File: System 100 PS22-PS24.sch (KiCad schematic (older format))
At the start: 39 parts, among them P1 CONN_01X01, P10 CONN_01X04, P11 CONN_01X06, P13 CONN_01X04, P2 CONN_01X01, P3 CONN_01X01, P4 CONN_01X01, P5 CONN_01X08, Q101 TIP31A, Q102 TIP31A, U101 LM723CN, U102 LM723CN

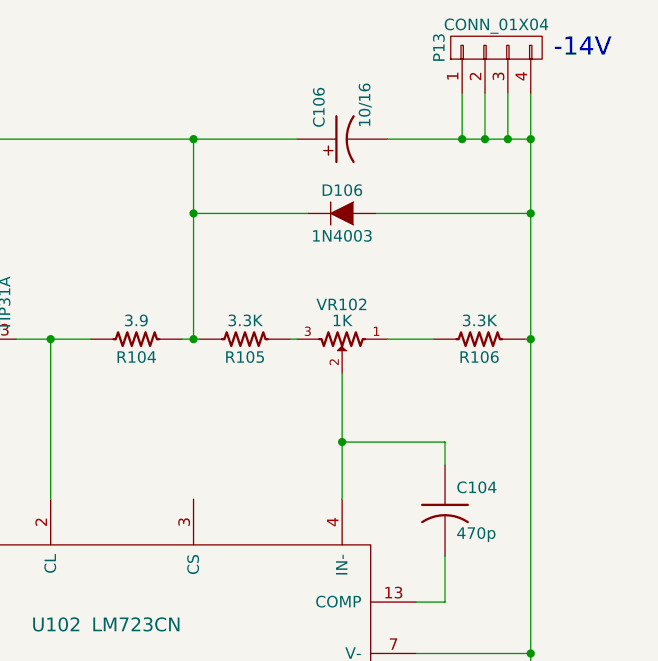
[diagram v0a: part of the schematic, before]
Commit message: routed
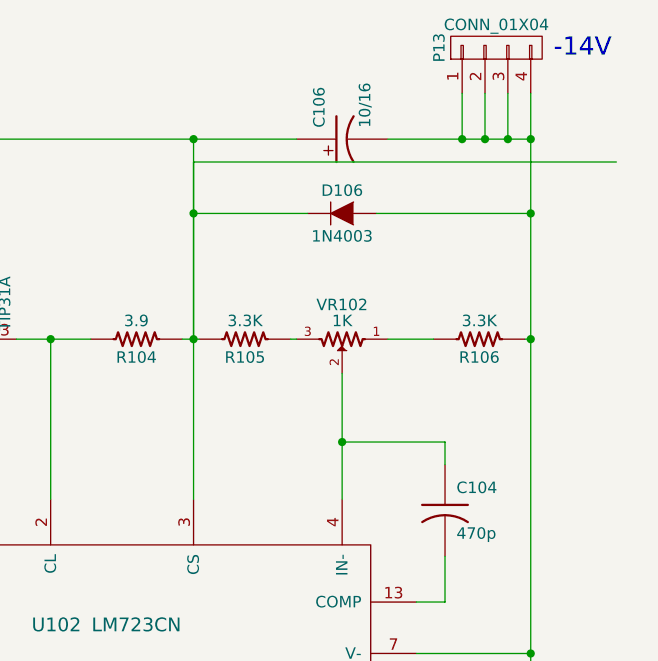
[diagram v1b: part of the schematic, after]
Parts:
- P1, P2, P3, P4: footprint (none) -> Pin_Headers:Pin_Header_Straight_1x01
- P10, P13: footprint (none) -> Pin_Headers:Pin_Header_Straight_1x04
- P11: footprint (none) -> Pin_Headers:Pin_Header_Straight_2x03
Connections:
- net GND: now also U102.3 (CS)
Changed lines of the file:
@@
 F 0 "P2" H 3100 6825 50  0000 C CNN
 F 1 "CONN_01X01" V 3200 6725 50  0000 C CNN
-F 2 "" H 3100 6725 60  0001 C CNN
+F 2 "Pin_Headers:Pin_Header_Straight_1x01" H 3100 6725 60  0001 C CNN
 F 3 "" H 3100 6725 60  0000 C CNN
 	1    3100 6725
@@
 F 0 "P3" H 2500 6825 50  0000 C CNN
 F 1 "CONN_01X01" V 2600 6725 50  0000 C CNN
-F 2 "" H 2500 6725 60  0001 C CNN
+F 2 "Pin_Headers:Pin_Header_Straight_1x01" H 2500 6725 60  0001 C CNN
 F 3 "" H 2500 6725 60  0000 C CNN
 	1    2500 6725
@@
 F 0 "P10" H 2675 425 50  0000 C CNN
 F 1 "CONN_01X04" V 2775 750 50  0000 C CNN
-F 2 "" H 2675 750 60  0001 C CNN
+F 2 "Pin_Headers:Pin_Header_Straight_1x04" H 2675 750 60  0001 C CNN
 F 3 "" H 2675 750 60  0000 C CNN
 	1    2675 750
@@
 F 0 "P11" H 4550 425 50  0000 C CNN
 F 1 "CONN_01X06" V 4650 775 50  0000 C CNN
-F 2 "" H 4550 775 60  0001 C CNN
+F 2 "Pin_Headers:Pin_Header_Straight_2x03" H 4550 775 60  0001 C CNN
 F 3 "" H 4550 775 60  0000 C CNN
 	1    4550 775
@@
 F 0 "P1" H 6450 6825 50  0000 C CNN
 F 1 "CONN_01X01" V 6550 6725 50  0000 C CNN
-F 2 "" H 6450 6725 60  0001 C CNN
+F 2 "Pin_Headers:Pin_Header_Straight_1x01" H 6450 6725 60  0001 C CNN
 F 3 "" H 6450 6725 60  0000 C CNN
 	1    6450 6725
@@
 F 0 "P4" H 5850 6825 50  0000 C CNN
 F 1 "CONN_01X01" V 5950 6725 50  0000 C CNN
-F 2 "" H 5850 6725 60  0001 C CNN
+F 2 "Pin_Headers:Pin_Header_Straight_1x01" H 5850 6725 60  0001 C CNN
 F 3 "" H 5850 6725 60  0000 C CNN
 	1    5850 6725
@@
 F 0 "P13" H 7500 1000 50  0000 C CNN
 F 1 "CONN_01X04" V 7600 750 50  0000 C CNN
-F 2 "" H 7500 750 60  0001 C CNN
+F 2 "Pin_Headers:Pin_Header_Straight_1x04" H 7500 750 60  0001 C CNN
 F 3 "" H 7500 750 60  0000 C CNN
 	1    7500 750
@@
 Wire Wire Line
 	6175 1150 6175 2025
+Wire Wire Line
+	8025 1250 6175 1250
+Wire Wire Line
+	6175 1250 6175 2725
 $EndSCHEMATC
